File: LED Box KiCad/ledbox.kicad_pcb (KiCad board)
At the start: 2 copper layers, 80 x 50 mm, 131 parts, among them CON401 AVR_ISP, J201 Bus, J301 IR LED, J302 Button, J401 Power, J402 Power, J403 Power, J404 Port D, J405 Port B, J406 Port C, J407 ADC6, J408 ADC7, J501 6.5V-12V, J502 5V, SW301 Reset, SW302 Push 1, SW303 Push 2, U201 ST485C, U301 ULN2003, U401 ATMEGA88-20AU, U501 AZ1117-5.0, Y401 DNP/20MHz

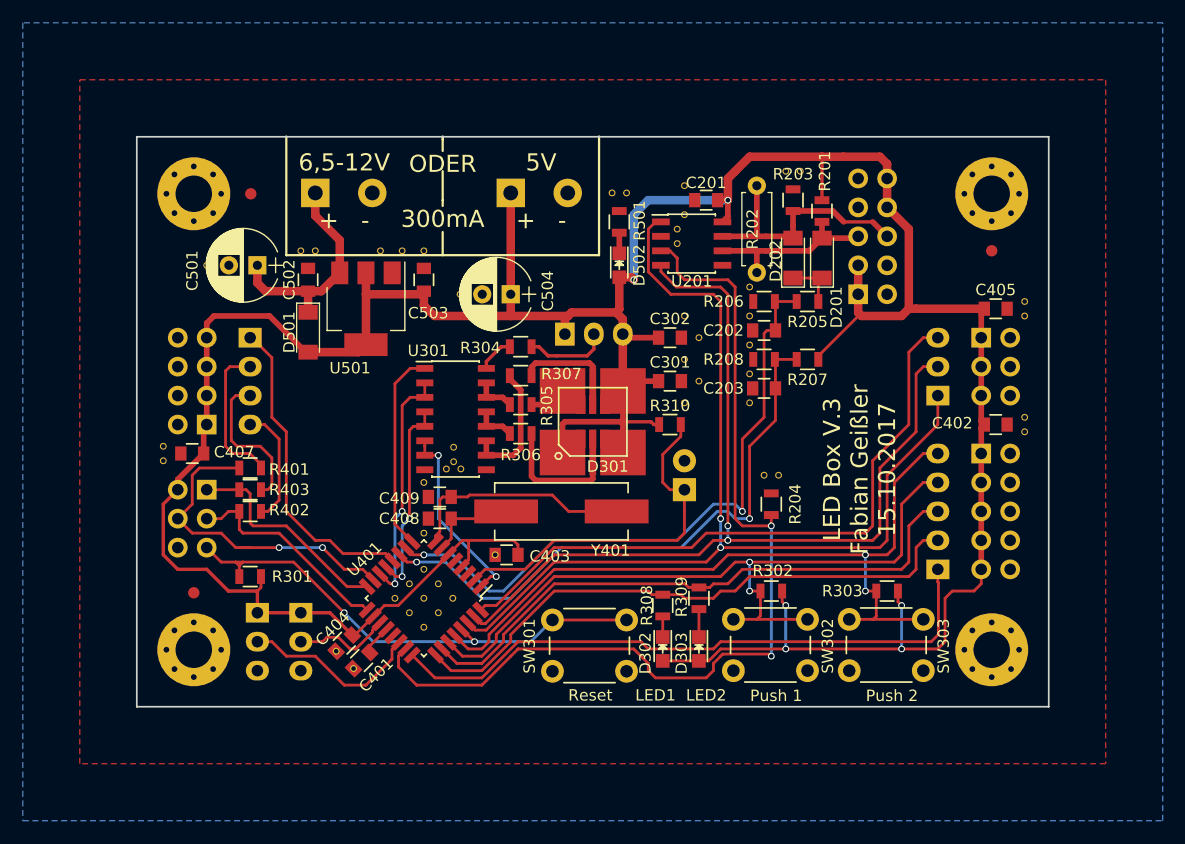
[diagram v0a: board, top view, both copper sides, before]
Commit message: Kleine Veränderungen
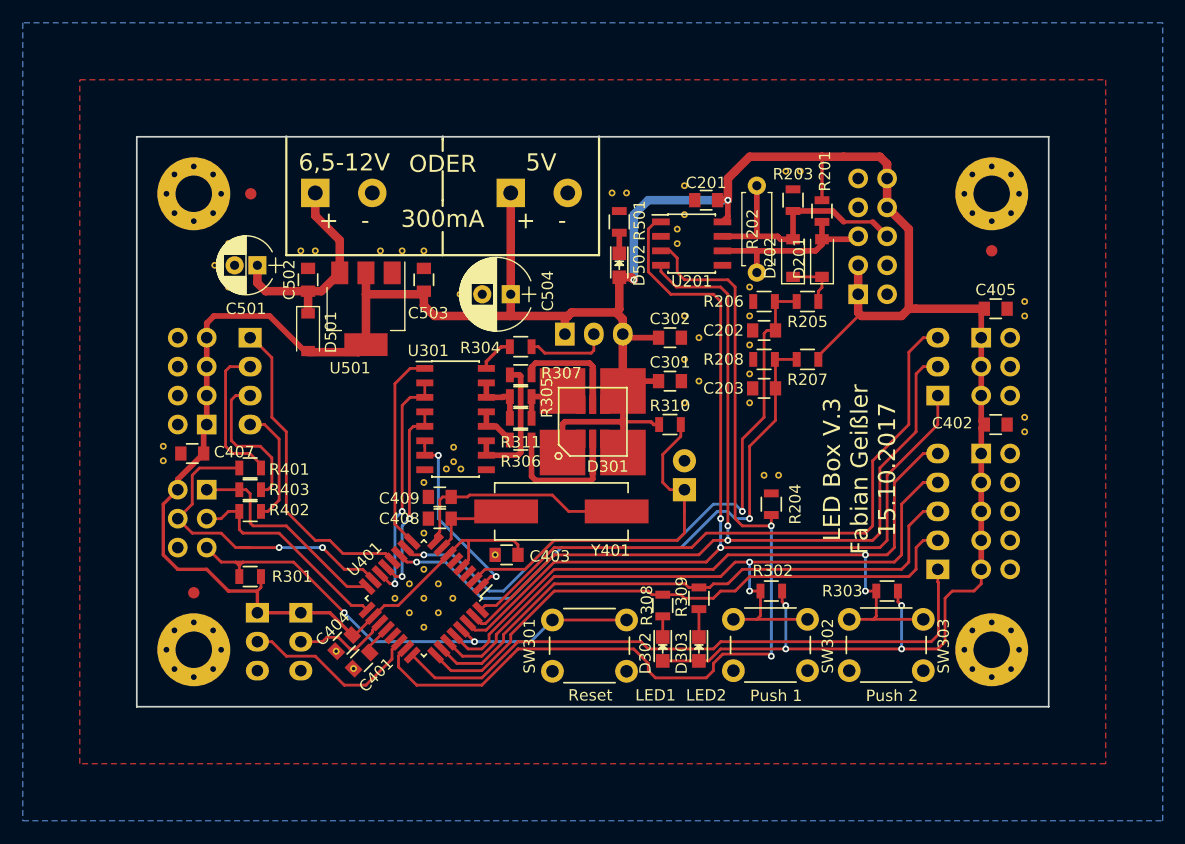
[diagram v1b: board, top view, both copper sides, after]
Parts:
- added R311: 82, Resistors_SMD:R_0805, F.Cu at (143.7, 99.7)
- C501: footprint Capacitors_THT:CP_Radial_D6.3mm_P2.50mm -> Capacitors_THT:CP_Radial_D5.0mm_P2.00mm
- D201, D202, D501: footprint Diodes_SMD:D_MiniMELF -> Diodes_SMD:D_SOD-123
- R305: value 42 -> 82
- moved R305 0.70 mm to (143.7, 97.8)
- moved REF** 0.70 mm to (116.8, 86.3)
- moved R306 0.56 mm to (143.7, 101.6)
- moved R307 0.07 mm to (143.7, 95.9)
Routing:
- net Net-(R305-Pad2): track 3.60 -> 5.27 mm
- net Net-(D301-Pad6): track 3.21 -> 4.83 mm
- net Net-(R307-Pad2): track 11.3 -> 12.1 mm
- net /Bus/COMM_A: track 15.8 -> 16.4 mm
- net Net-(D301-Pad2): track 11.6 -> 11.1 mm
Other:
- net class Default: via_dia 0.7 -> 0.6; via_drill 0.4 -> 0.3
